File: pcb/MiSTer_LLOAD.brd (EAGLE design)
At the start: 100 x 80 mm, 26 parts, among them IC3 REG1117, K1 692121030100

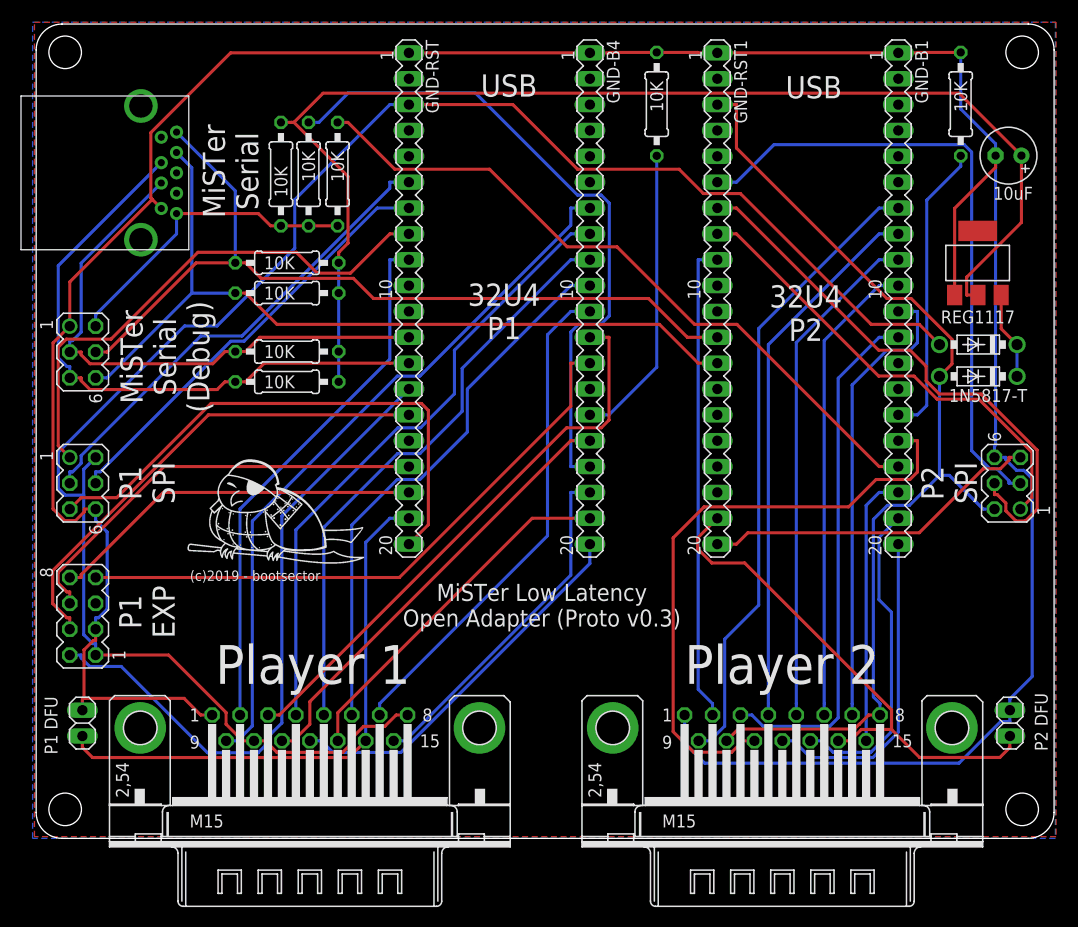
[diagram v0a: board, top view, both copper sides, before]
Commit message: Promoting LLOAD PCB to v1.0
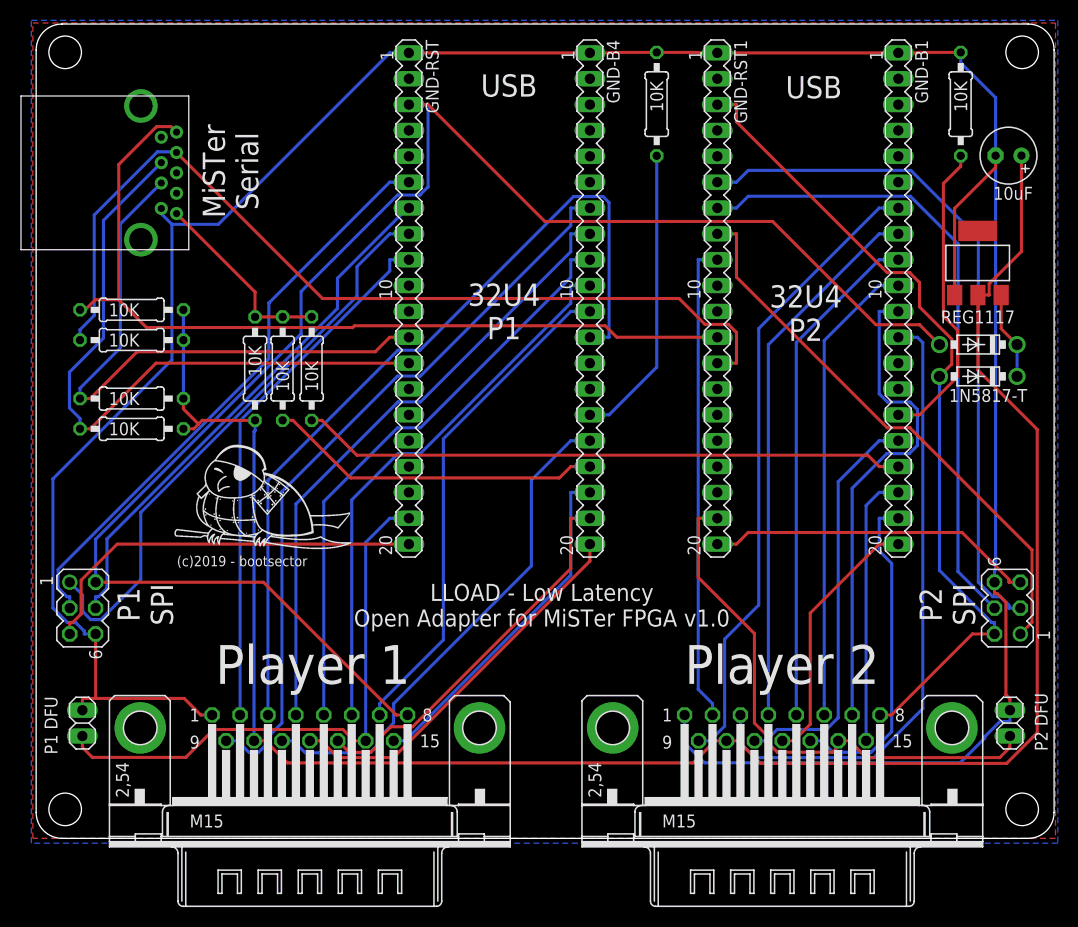
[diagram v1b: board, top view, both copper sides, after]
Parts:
- removed SV2: (no value), con-lstb:MA04-2
- removed SV4: (no value), con-lstb:MA03-2
- moved R7 19.3 mm to (21.5, 46.1), turned to 270 degrees
- moved R8 19.3 mm to (24.2, 46.1), turned to 90 degrees
- moved R9 19.3 mm to (27.1, 46.1), turned to 90 degrees
- moved R2 15.9 mm to (9.39, 43.2)
- moved R3 15.9 mm to (9.39, 40.2)
- moved R5 15.9 mm to (9.39, 51.9)
- moved R6 15.9 mm to (9.39, 49.0)
- moved SV1 12.3 mm to (4.57, 22.6)
- moved SV3 12.3 mm to (95.4, 22.6)
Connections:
- net 3V3: now also X1.10, X2.10
- net D0: no longer SV4.3
- net D1: no longer SV4.5
- net D2: no longer SV2.2
- net D3: no longer SV2.4
- net D5: no longer SV2.6
- net D6: no longer SV2.8
- net F7: no longer SV2.7
- net GND: no longer SV2.3, SV4.1
- net LL_ENABLE: no longer SV4.2
- net P1_VCC: no longer SV2.1, X2.10
- net P2_D0: no longer SV4.4
- net P2_D1: no longer SV4.6
- net P2_VCC: no longer X1.10
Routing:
- net 3V3: track 121.6 -> 193.2 mm
- net D2: track 64.5 -> 0.00 mm
- net F7: track 59.8 -> 0.00 mm
- net D3: track 47.9 -> 0.00 mm
- net D5: track 42.4 -> 0.00 mm
- net D6: track 36.9 -> 0.00 mm
- net C6: track 65.9 -> 33.0 mm
- net F6: track 55.5 -> 83.5 mm
- net P2_C7: track 60.0 -> 39.9 mm
- net P2_VCC: track 99.7 -> 81.4 mm
- net P1_VCC: track 177.2 -> 161.6 mm
- net RST: track 53.7 -> 39.6 mm
- net GND: track 288.7 -> 276.0 mm
- net LL_ENABLE: track 30.7 -> 18.9 mm
- net B1: track 47.0 -> 57.9 mm
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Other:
- board text added: "LLOAD - Low Latency Open Adapter for MiSTer FPGA v1.0"
- board text removed: "MiSTer Low Latency Open Adapter (Proto v0.3)"
- board text removed: "MiSTer Serial (Debug)"
- board text removed: "P1 EXP"
